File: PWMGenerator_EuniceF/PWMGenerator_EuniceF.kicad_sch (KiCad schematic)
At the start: 12 parts, among them J1 Conn_01x03_Pin, Q1 NPN, Q2 NPN, Q3 PNP, Q4 PNP, SW1 SW_SPST, U1 LM7805_TO220, U2 LM339

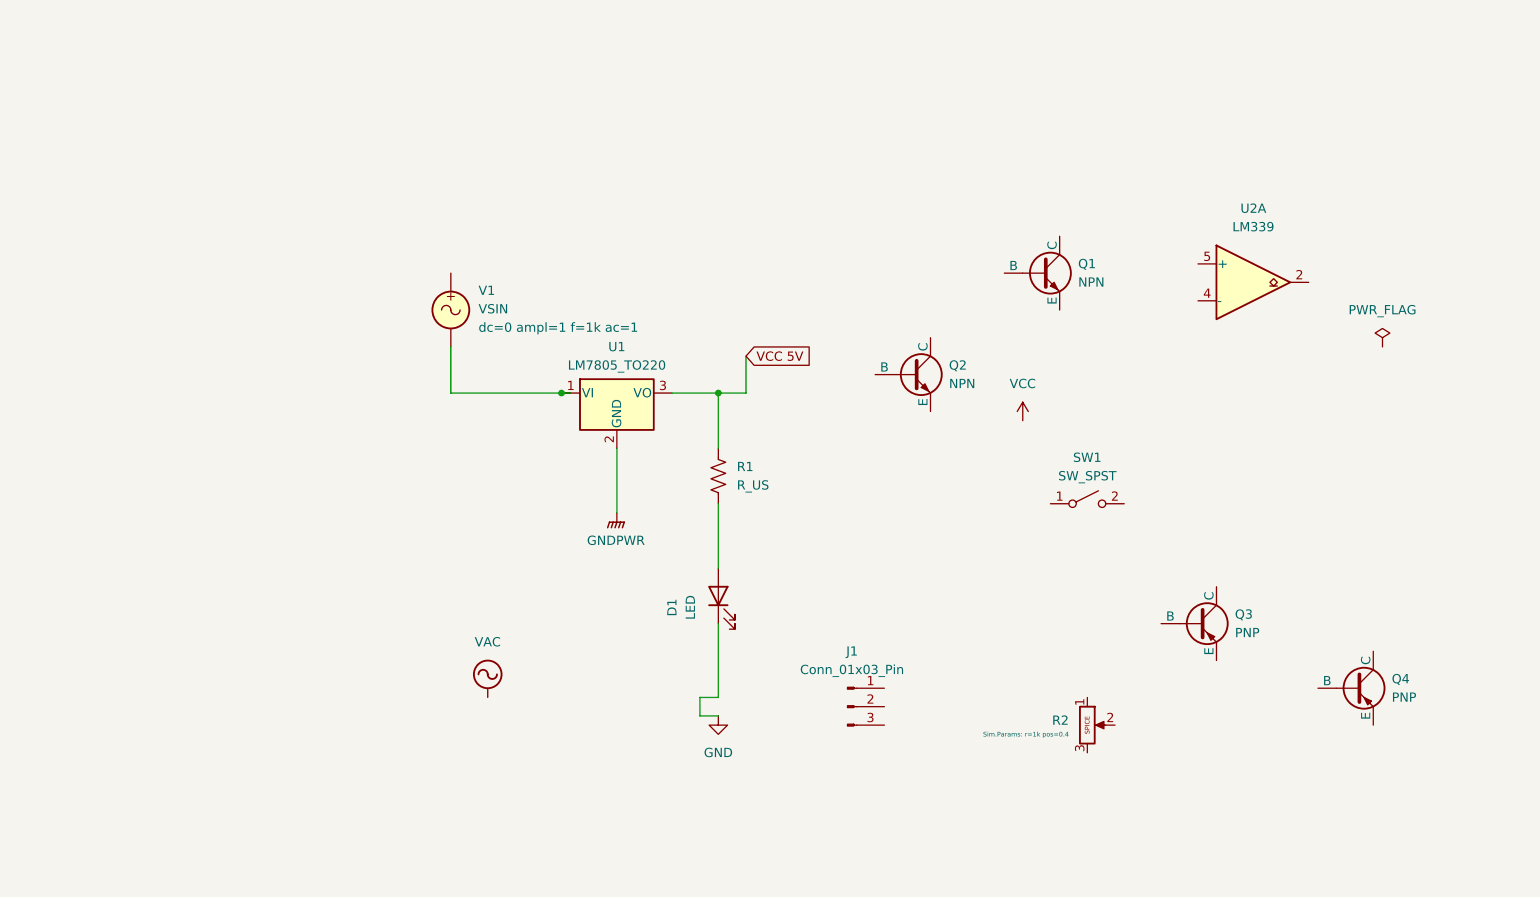
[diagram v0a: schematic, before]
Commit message: PWMGenerator
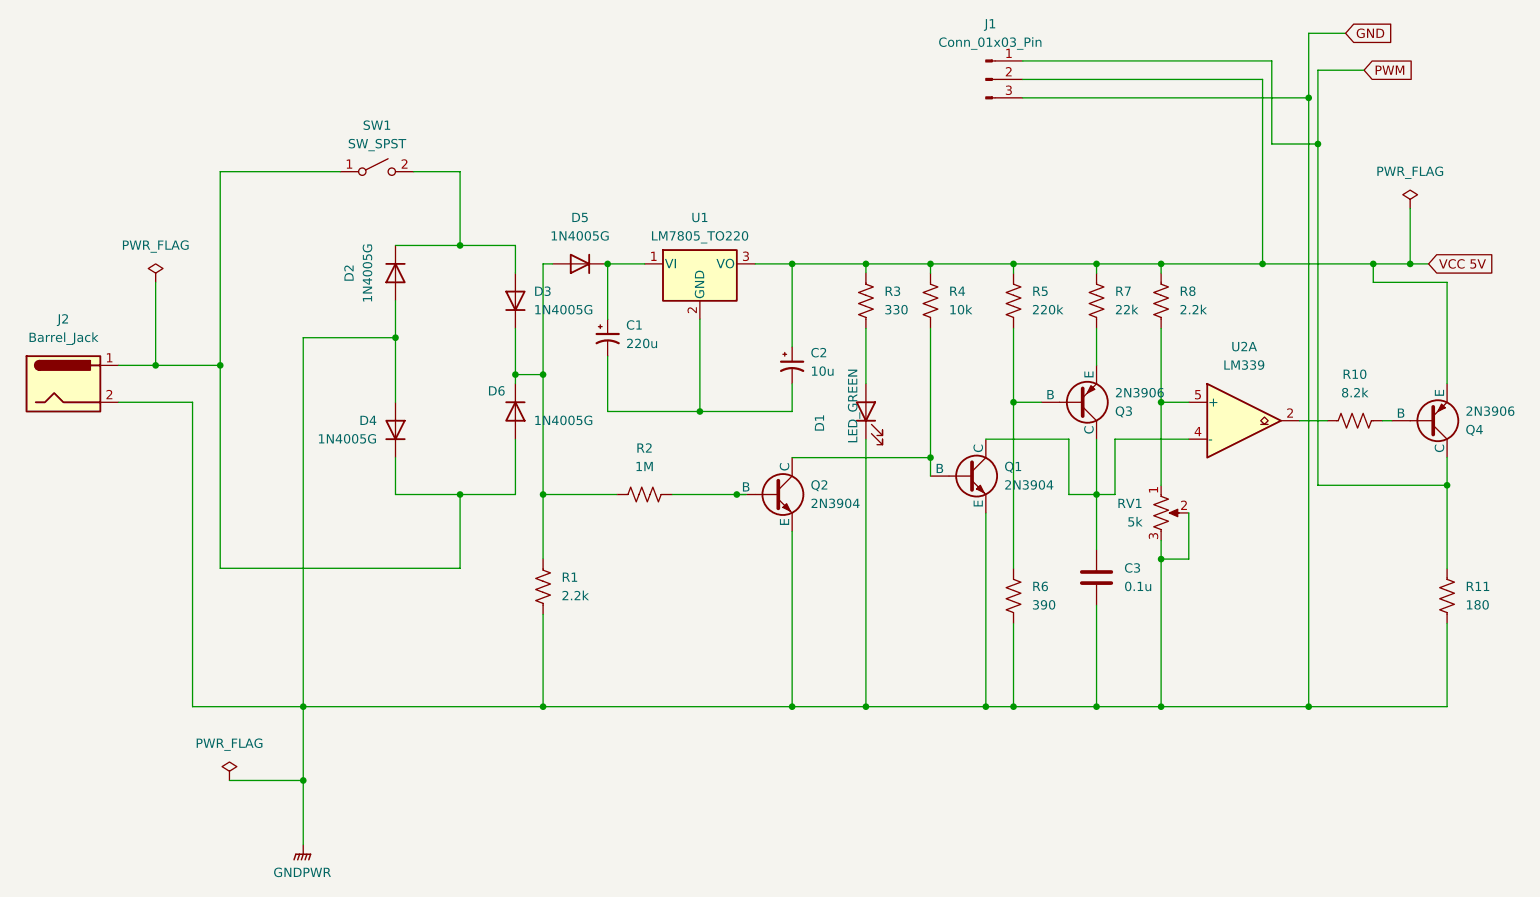
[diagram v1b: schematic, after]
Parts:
- removed R2: Potentiometer, symbol Simulation_SPICE:Potentiometer
- removed V1: VSIN, symbol Simulation_SPICE:VSIN
- added C1: 220u, Capacitor_THT:CP_Radial_D10.0mm_P5.00mm_P7.50mm, symbol Device:C_Polarized_Small_US
- added C2: 10u, Capacitor_THT:CP_Radial_D10.0mm_P5.00mm_P7.50mm, symbol Device:C_Polarized_Small_US
- added C3: 0.1u, Capacitor_SMD:C_0805_2012Metric, symbol Device:C
- added D2, D4, D5, D6: 1N4005G, Diode_SMD:D_0805_2012Metric, symbol Diode:1N4005
- added D3: 1N4005G, Diode_THT:D_DO-41_SOD81_P10.16mm_Horizontal, symbol Diode:1N4005
- added J2: Barrel_Jack, Connector_BarrelJack:BarrelJack_CUI_PJ-063AH_Horizontal, symbol Connector:Barrel_Jack
- added R10: 8.2k, Resistor_SMD:R_0805_2012Metric, symbol Device:R_US
- added R11: 180, Resistor_SMD:R_0805_2012Metric, symbol Device:R_US
- added R2: 1M, Resistor_SMD:R_0805_2012Metric, symbol Device:R_US
- added R3: 330, Resistor_SMD:R_0805_2012Metric, symbol Device:R_US
- added R4: 10k, Resistor_SMD:R_0805_2012Metric, symbol Device:R_US
- added R5: 220k, Resistor_SMD:R_0805_2012Metric, symbol Device:R_US
- added R6: 390, Resistor_SMD:R_0805_2012Metric, symbol Device:R_US
- added R7: 22k, Resistor_SMD:R_0805_2012Metric, symbol Device:R_US
- added R8: 2.2k, Resistor_SMD:R_0805_2012Metric, symbol Device:R_US
- added RV1: 5k, Potentiometer_THT:Potentiometer_ACP_CA14-H2,5_Horizontal, symbol Device:R_Potentiometer_US
- D1: value LED -> LED_GREEN; footprint (none) -> LED_THT:LED_D5.0mm_GREEN
- J1: footprint (none) -> Connector_PinHeader_2.54mm:PinHeader_1x03_P2.54mm_Horizontal
- Q1, Q2: value NPN -> 2N3904; footprint (none) -> Package_TO_SOT_SMD:SOT-23
- Q3, Q4: value PNP -> 2N3906; footprint (none) -> Package_TO_SOT_SMD:SOT-23
- R1: value R_US -> 2.2k; footprint (none) -> Resistor_SMD:R_0805_2012Metric
- SW1: footprint (none) -> Button_Switch_SMD:SW_DIP_SPSTx01_Slide_6.7x4.1mm_W6.73mm_P2.54mm_LowProfile_JPin
- U1: footprint Package_TO_SOT_THT:TO-220-3_Vertical -> Package_TO_SOT_THT:TO-220-3_Horizontal_TabDown
- U2: footprint (none) -> Package_SO:SOIC-14_3.9x8.7mm_P1.27mm
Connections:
- net GND is gone; now on net GNDPWR: D1.1 (K)
- net GNDPWR: now also J1.3 (Pin_3), Q1.3 (E), Q2.3 (E), R1.2, C3.2, D2.2 (A), D4.2 (A), J2.2, R11.2, R6.2, RV1.2, RV1.3; no longer U1.2 (GND)
- net VCC 5V: now also J1.2 (Pin_2), Q4.3 (E), C2.1, R3.1, R4.1, R5.1, R7.1, R8.1; no longer R1.1
- net at SW1.1 (A): now also D4.1 (K), D6.2 (A), J2.1
- net at SW1.2 (B): now also D2.1 (K), D3.2 (A)
- net at U2.2: now also R10.1
- net at U2.4 (-): now also Q1.1 (C), Q3.1 (C), C3.1
- net at U2.5 (+): now also R8.2, RV1.1
- net at D1.2 (A): now also R3.2; no longer R1.2
- net at Q1.2 (B): now also Q2.1 (C), R4.2
- net at Q3.2 (B): now also R5.2, R6.1
- net at Q3.3 (E): now also R7.2
- net at U1.1 (VI): now also C1.1, D5.1 (K)
- net PWM: now reaches Q4.1 (C)
- net PWM: now also J1.1 (Pin_1), R11.1
- net at Q4.2 (B): now also R10.2
- net at Q2.2 (B): now also R2.2
- new net: D3.1 (K), D5.2 (A), D6.1 (K), R1.1, R2.1
- new net: C1.2, C2.2, U1.2 (GND)
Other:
- moved on the sheet: D1, J1, Q1, Q2, Q3, Q4, SW1, U1, U2A
